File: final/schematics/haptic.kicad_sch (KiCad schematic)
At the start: 11 parts, among them U4 DRV2605LDGST, U5 DRV2605LDGST, U6 DRV2605LDGST

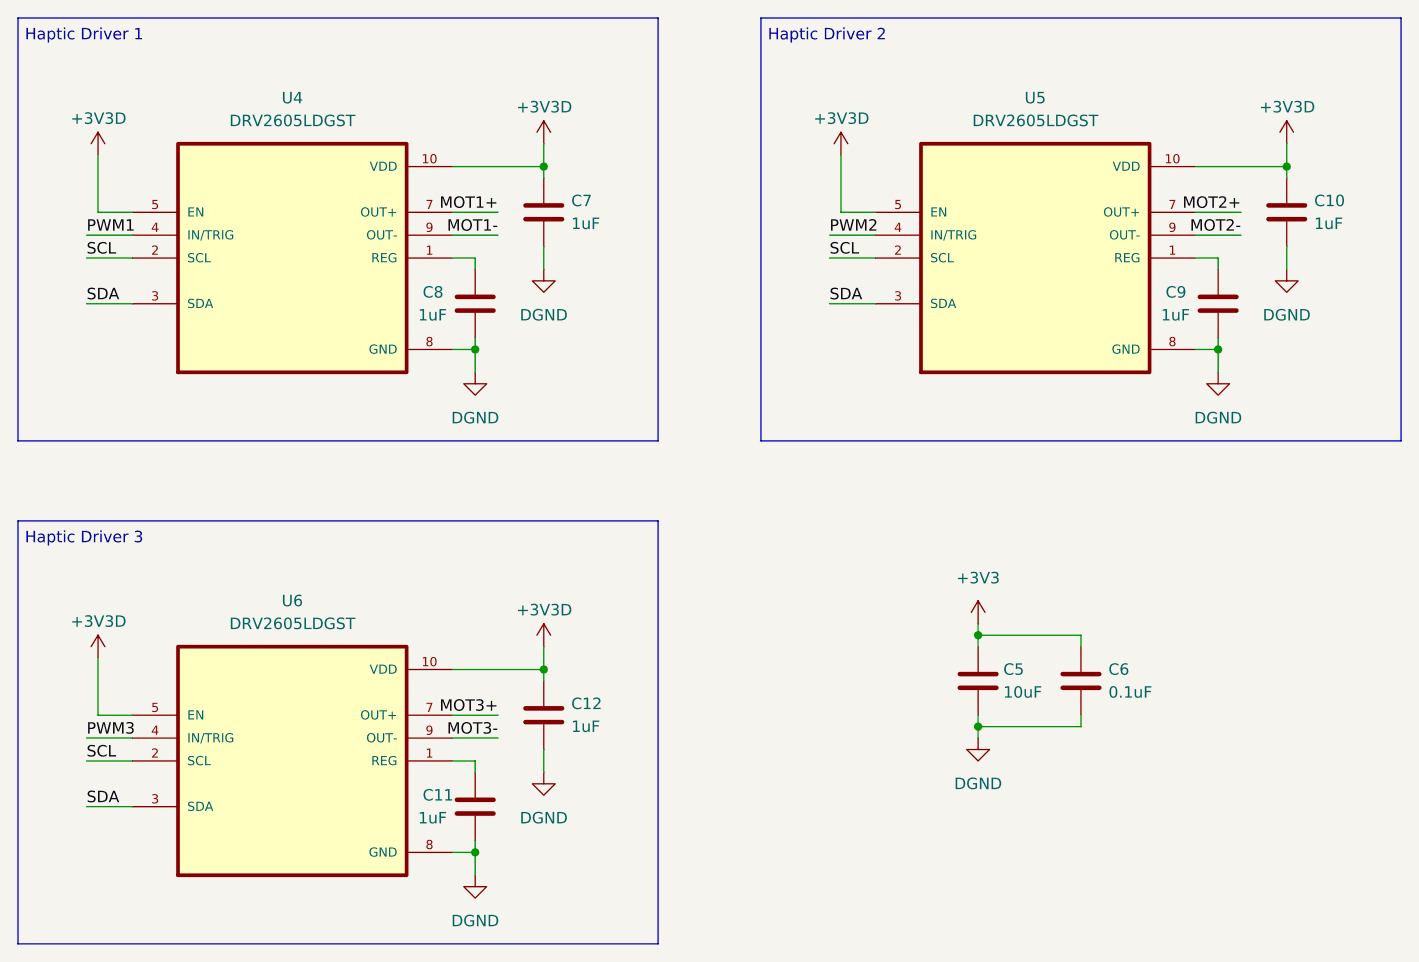
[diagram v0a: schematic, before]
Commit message: finishing
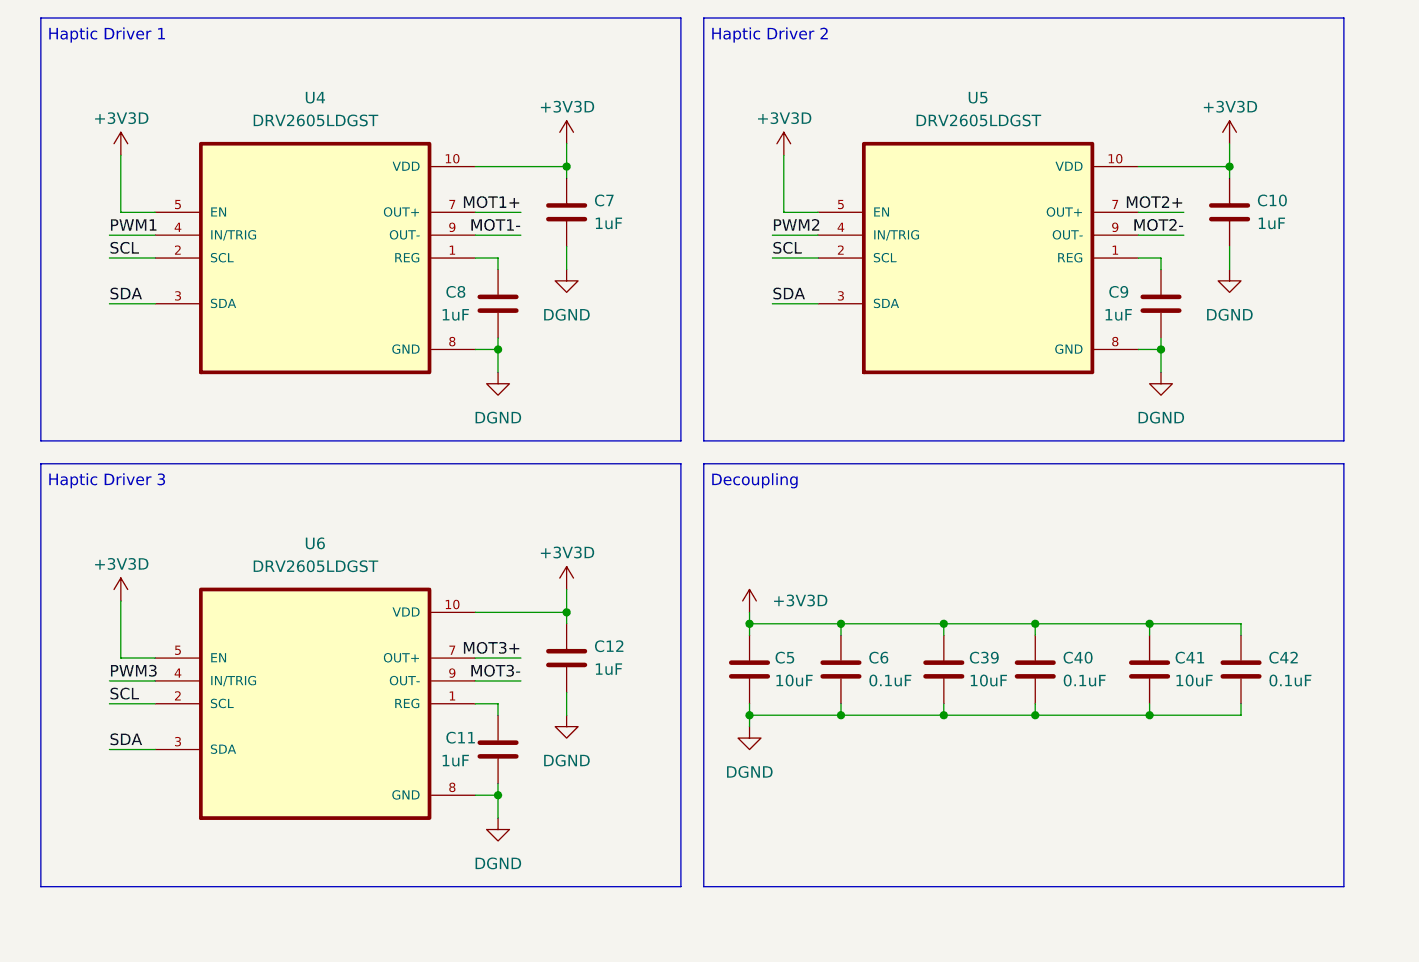
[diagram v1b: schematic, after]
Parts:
- added C39, C41: 10uF, Capacitor_SMD:C_0603_1608Metric, symbol Device:C
- added C40, C42: 0.1uF, Capacitor_SMD:C_0603_1608Metric, symbol Device:C
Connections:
- net +3V3 is gone; now on net +3V3D: C5.1, C6.1
- net +3V3D: now also C39.1, C40.1, C41.1, C42.1
- net DGND: now also C39.2, C40.2, C41.2, C42.2
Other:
- note added: "Decoupling"
- moved on the sheet: C10, C11, C12, C5, C6, C7, C8, C9, U4, U5, U6
